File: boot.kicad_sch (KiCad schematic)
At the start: 1 part

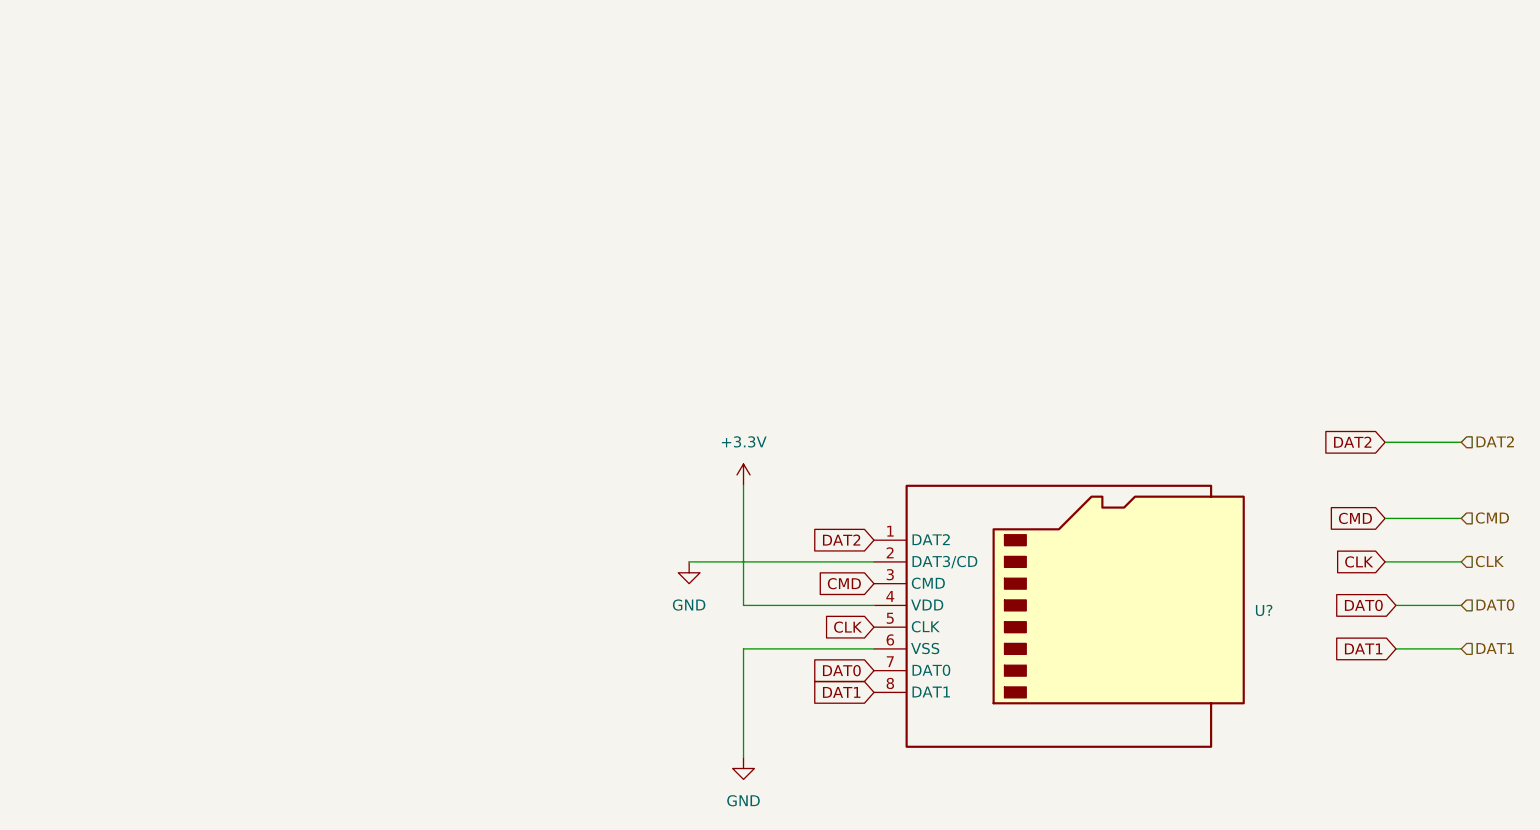
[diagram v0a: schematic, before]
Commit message: Add files via upload
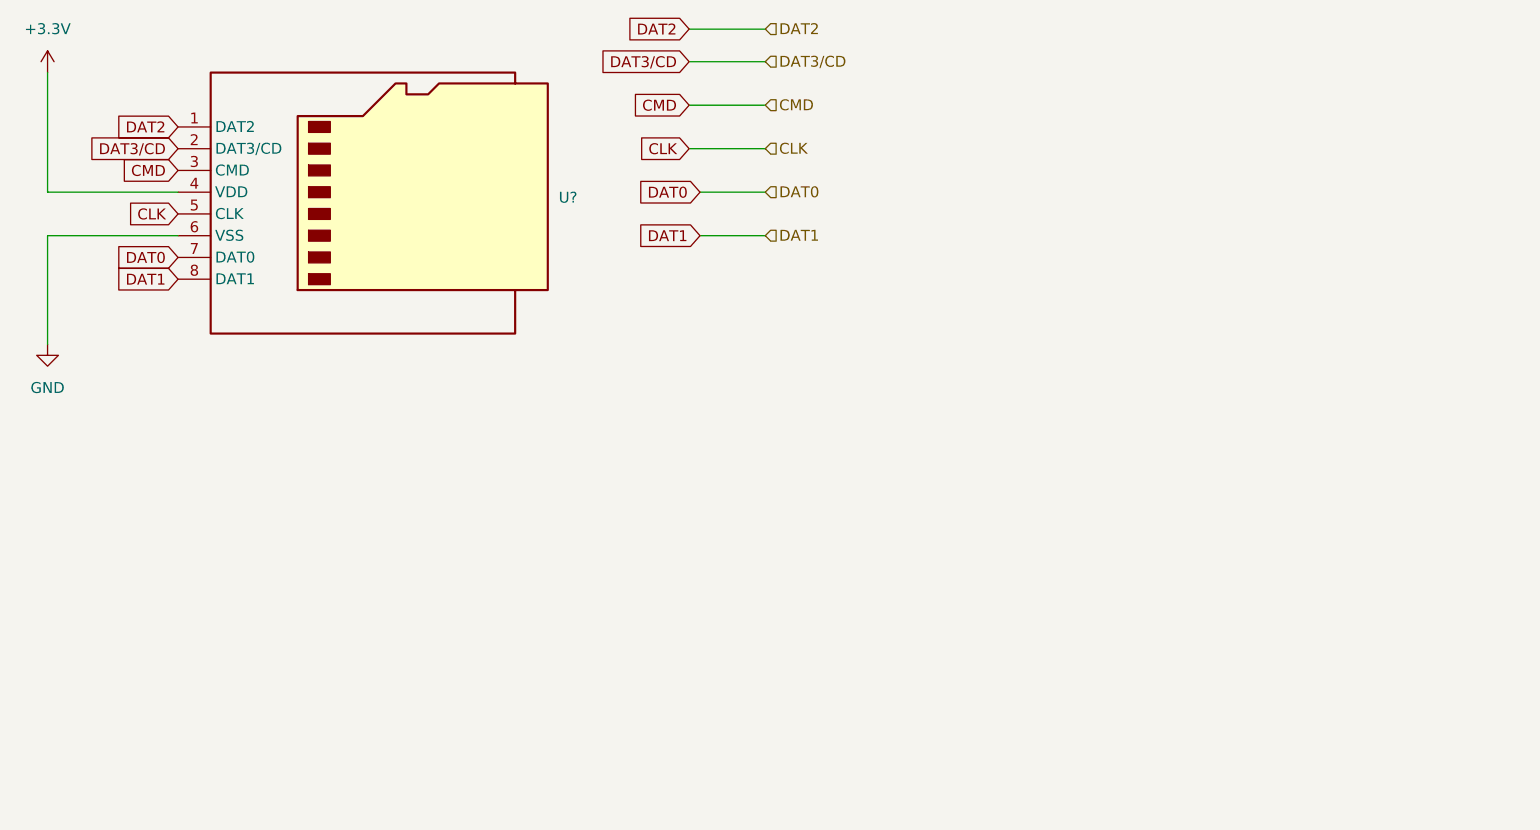
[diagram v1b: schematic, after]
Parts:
- removed U?: ~, symbol Aftx07:MSD-4-A
- added U?: ~, symbol Aftx07:MSD-4-A
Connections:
- net +3.3V: now also U?.4 (VDD)
- net CLK: now also U?.5 (CLK)
- net CMD: now also U?.3 (CMD)
- net DAT0: now also U?.7 (DAT0)
- net DAT1: now also U?.8 (DAT1)
- net DAT2: now also U?.1 (DAT2)
- net GND: now also U?.6 (VSS)
- new net DAT3/CD: U?.2 (DAT3/CD)
